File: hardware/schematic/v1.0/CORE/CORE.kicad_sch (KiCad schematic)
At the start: 79 parts, among them J1 Conn_01x03_Socket, J10 USB_C_Receptacle_USB2.0_16P, J11 Conn_01x06_Socket, J2 Conn_Coaxial, J3 Conn_Coaxial, J4 Conn_Coaxial, J5 Conn_Coaxial, J6 Conn_Coaxial, J7 Conn_Coaxial, J8 Conn_Coaxial, J9 Conn_Coaxial, M1 ZYNQ7010&7020, U1 TXS02612RTWR, U2 SP3232, U3 SD_Card, U4 AMS1117-2.5, U5 AMS1117-1.8

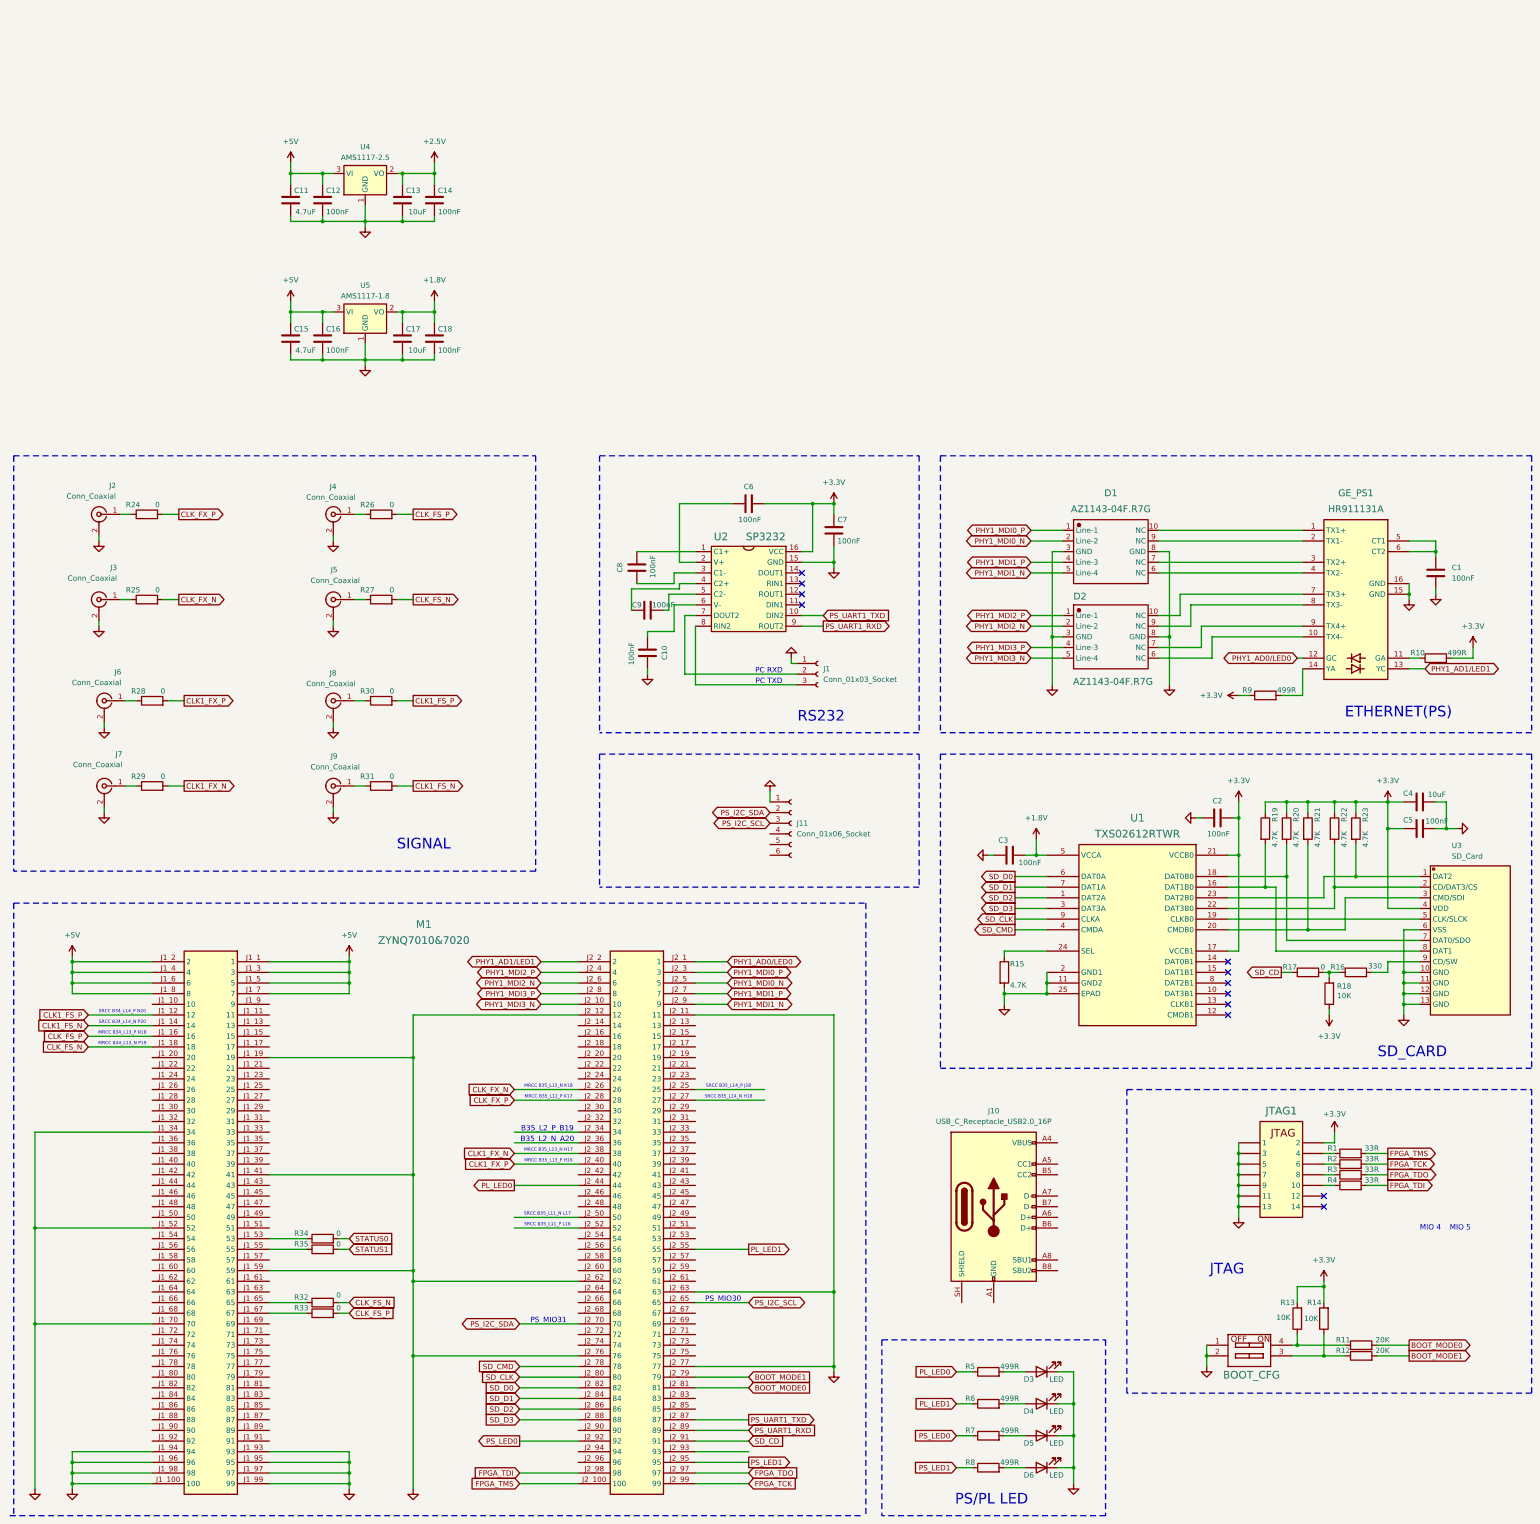
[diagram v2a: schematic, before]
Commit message: sch update
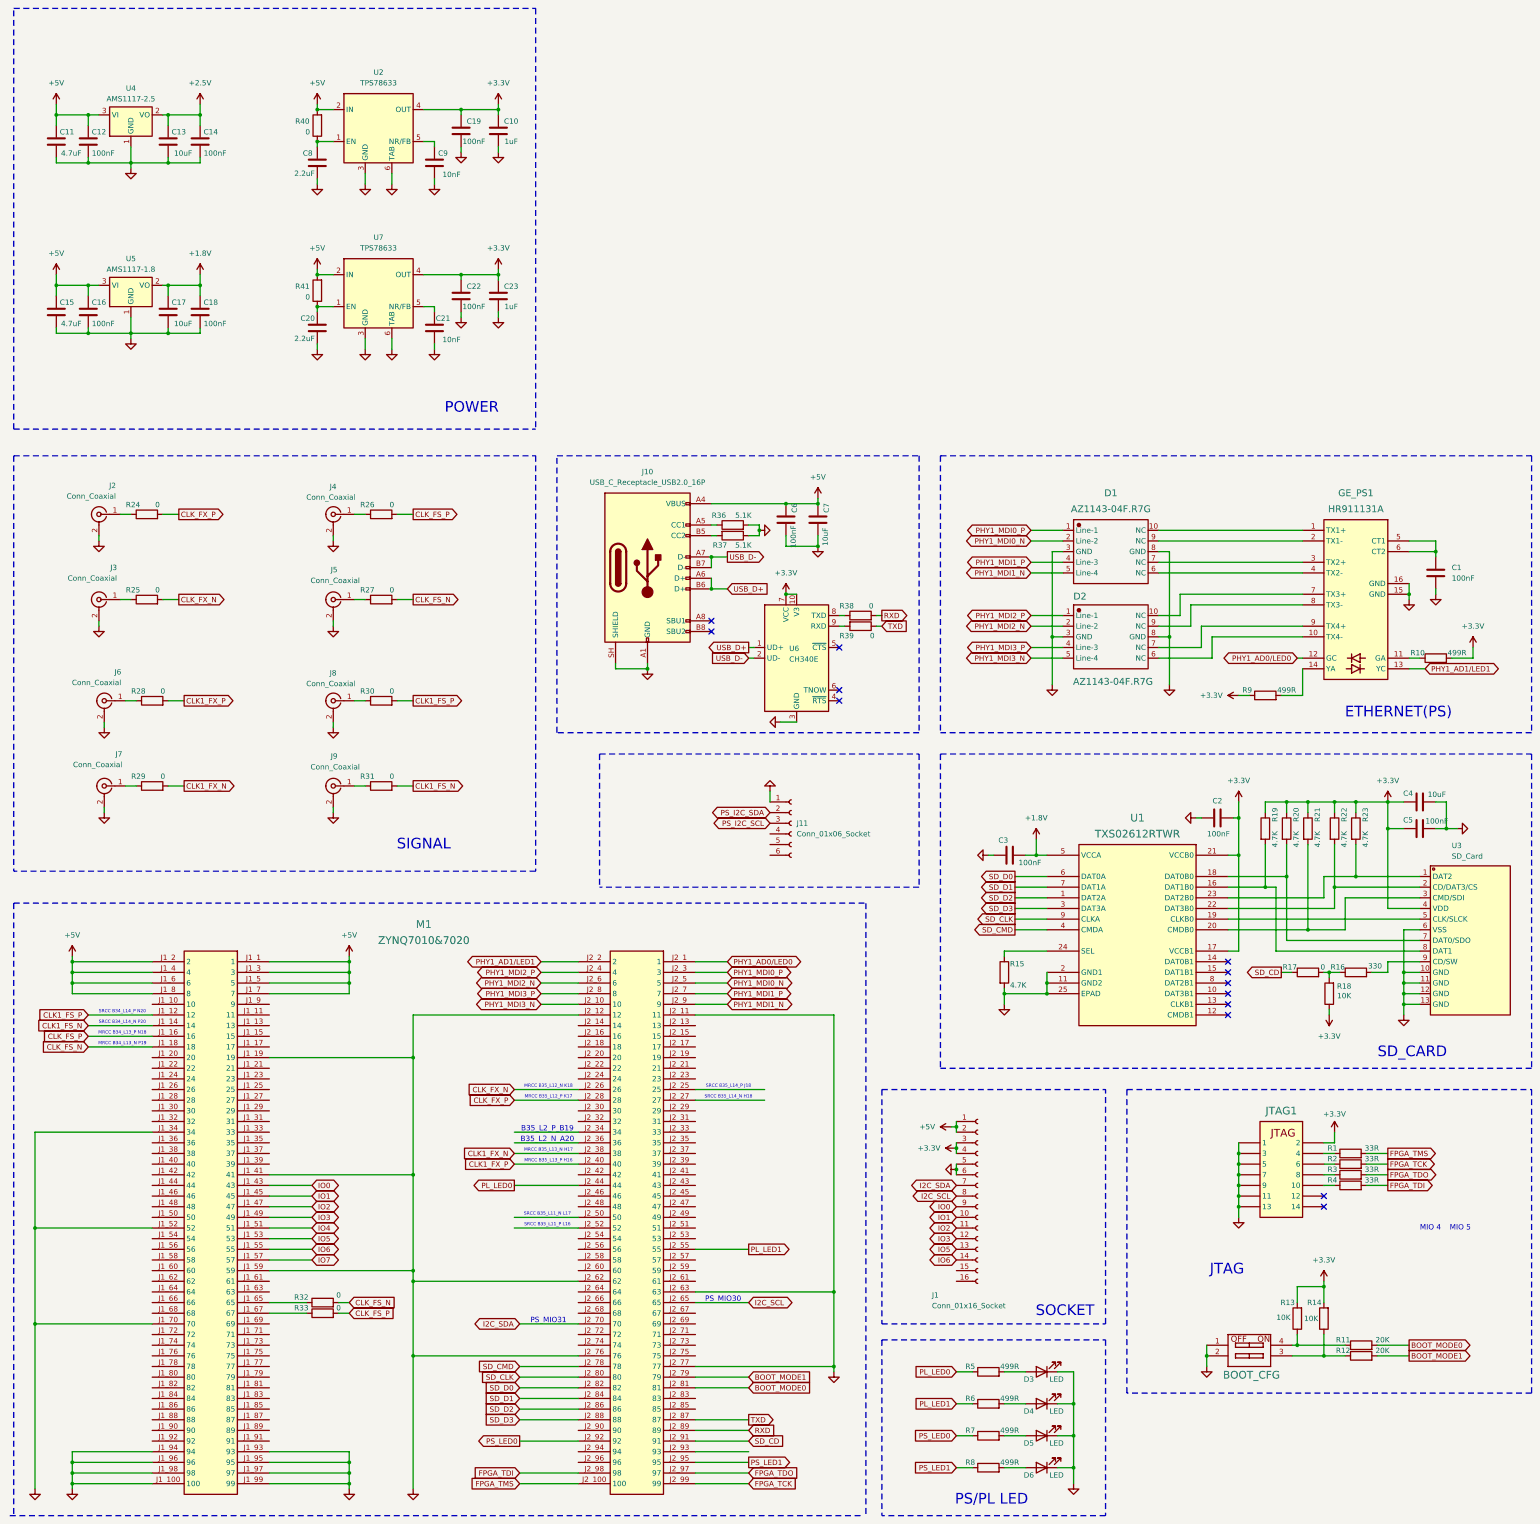
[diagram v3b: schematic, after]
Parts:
- removed J1: Conn_01x03_Socket, Connector_PinHeader_2.54mm:PinHeader_1x03_P2.54mm_Vertical, symbol Connector:Conn_01x03_Socket
- removed R34, R35: 0, Resistor_SMD:R_0402_1005Metric, symbol Device:R
- removed U2: SP3232, Counter:SOP16M, symbol Counter:MAX3232
- added C19, C22: 100nF, Capacitor_SMD:C_0402_1005Metric, symbol Device:C
- added C20: 2.2uF, Capacitor_SMD:C_0402_1005Metric, symbol Device:C
- added C21: 10nF, Capacitor_SMD:C_0402_1005Metric, symbol Device:C
- added C23: 1uF, Capacitor_SMD:C_0402_1005Metric, symbol Device:C
- added J1: Conn_01x16_Socket, Connector_PinSocket_2.54mm:PinSocket_1x16_P2.54mm_Vertical, symbol Connector:Conn_01x16_Socket
- added R36, R37: 5.1K, Resistor_SMD:R_0402_1005Metric, symbol Device:R
- added R38, R39, R40, R41: 0, Resistor_SMD:R_0402_1005Metric, symbol Device:R
- added U2, U7: TPS78633, Package_TO_SOT_SMD:SOT-223-6, symbol Counter:TPS78633
- added U6: CH340E, Package_SO:MSOP-10_3x3mm_P0.5mm, symbol Interface_USB:CH340E
- C10: value 100nF -> 1uF
- C7: value 100nF -> 10uF
- C8: value 100nF -> 2.2uF
- C9: value 100nF -> 10nF
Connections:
- net +3.3V: now also C10.2, C19.2, C22.2, C23.2, J1.3 (Pin_3), J1.4 (Pin_4), U2.4 (OUT), U6.10 (V3), U6.7 (VCC), U7.4 (OUT); no longer C6.2, C7.2
- net +5V: now also C6.1, C7.1, J10.A4 (VBUS), J10.A9 (VBUS), J10.B4 (VBUS), J10.B9 (VBUS), J1.1 (Pin_1), J1.2 (Pin_2), R40.2, R41.2, U2.2 (IN), U7.2 (IN)
- net GND: now also C10.1, C6.2, C7.2, C8.1, C9.1, J10.A1 (GND), J10.A12 (GND), J10.B1 (GND), J10.B12 (GND), J10.SH (SHIELD), C19.1, C20.1, C21.1, C22.1, C23.1, J1.5 (Pin_5), J1.6 (Pin_6), R36.2, R37.1, U2.3 (GND), U2.6 (TAB), U6.3 (GND), U7.3 (GND), U7.6 (TAB); no longer C10.2, C7.1
- net PS_I2C_SCL: no longer M1.J2_65 (65)
- net PS_I2C_SDA: no longer M1.J2_70 (70)
- net IO0: now reaches M1.J1_43 (43)
- net IO0: now also J1.9 (Pin_9)
- net IO1: now reaches M1.J1_45 (45)
- net IO1: now also J1.10 (Pin_10)
- net IO2: now reaches M1.J1_47 (47)
- net IO2: now also J1.11 (Pin_11)
- net IO3: now reaches M1.J1_49 (49)
- net IO3: now also J1.12 (Pin_12)
- net IO4: now reaches M1.J1_51 (51)
- net IO5: now reaches M1.J1_53 (53)
- net IO5: now also J1.13 (Pin_13)
- net IO6: now reaches M1.J1_55 (55)
- net IO6: now also J1.14 (Pin_14)
- net IO7: now reaches M1.J1_57 (57)
- net at C8.2: now also R40.1, U2.1 (EN)
- net at J10.A5 (CC1): now also R36.1
- net USB_D+: now reaches J10.A6 (D+)
- net USB_D+: now also J10.B6 (D+), U6.1 (UD+)
- net USB_D-: now reaches J10.A7 (D-)
- net USB_D-: now also J10.B7 (D-), U6.2 (UD-)
- net at J10.B5 (CC2): now also R37.2
- net at C9.2: now also U2.5 (NR/FB)
- net PS_UART1_RXD renamed RXD
- net RXD: now also R38.2
- net PS_UART1_TXD renamed TXD
- net TXD: now also R39.1
- new net: C20.2, R41.1, U7.1 (EN)
- new net: R38.1, U6.8 (TXD)
- new net: R39.2, U6.9 (RXD)
- new net: C21.2, U7.5 (NR/FB)
- new net I2C_SCL: J1.8 (Pin_8), M1.J2_65 (65)
- new net I2C_SDA: J1.7 (Pin_7), M1.J2_70 (70)
- no-connect marks 12 -> 13
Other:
- note added: "POWER"
- note added: "SOCKET"
- note removed: "PC RXD"
- note removed: "PC TXD"
- note removed: "RS232"
- moved on the sheet: C11, C12, C13, C14, C15, C16, C17, C18, J10, U4, U5
